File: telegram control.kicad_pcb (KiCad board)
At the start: 2 copper layers, 85.5 x 56 mm, 15 parts, among them J1 Screw_Terminal_01x03, J2 Screw_Terminal_01x02, K1 SANYOU_SRD_Form_C, Q1 MMBT3904, U1 ESP32-C3_SUPERMINI_TH, U3 L7805

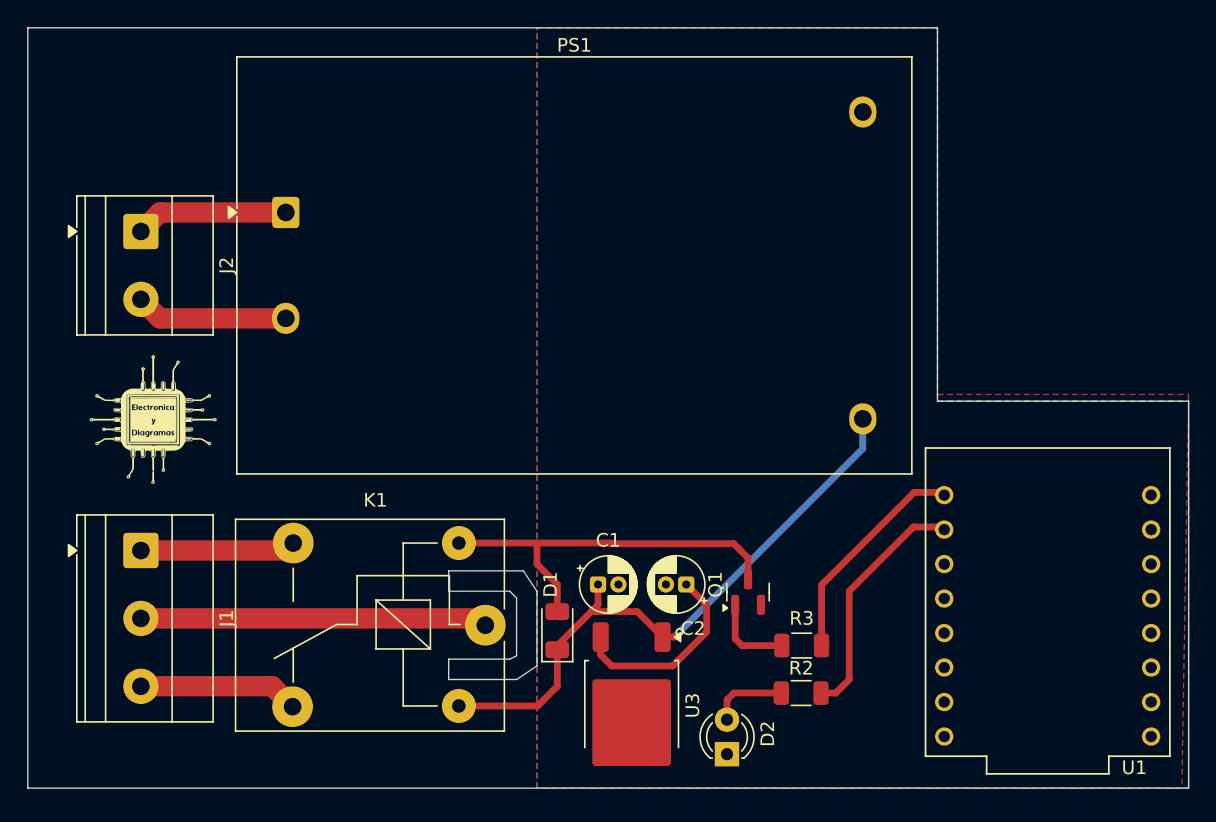
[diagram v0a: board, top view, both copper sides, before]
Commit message: telegram_control
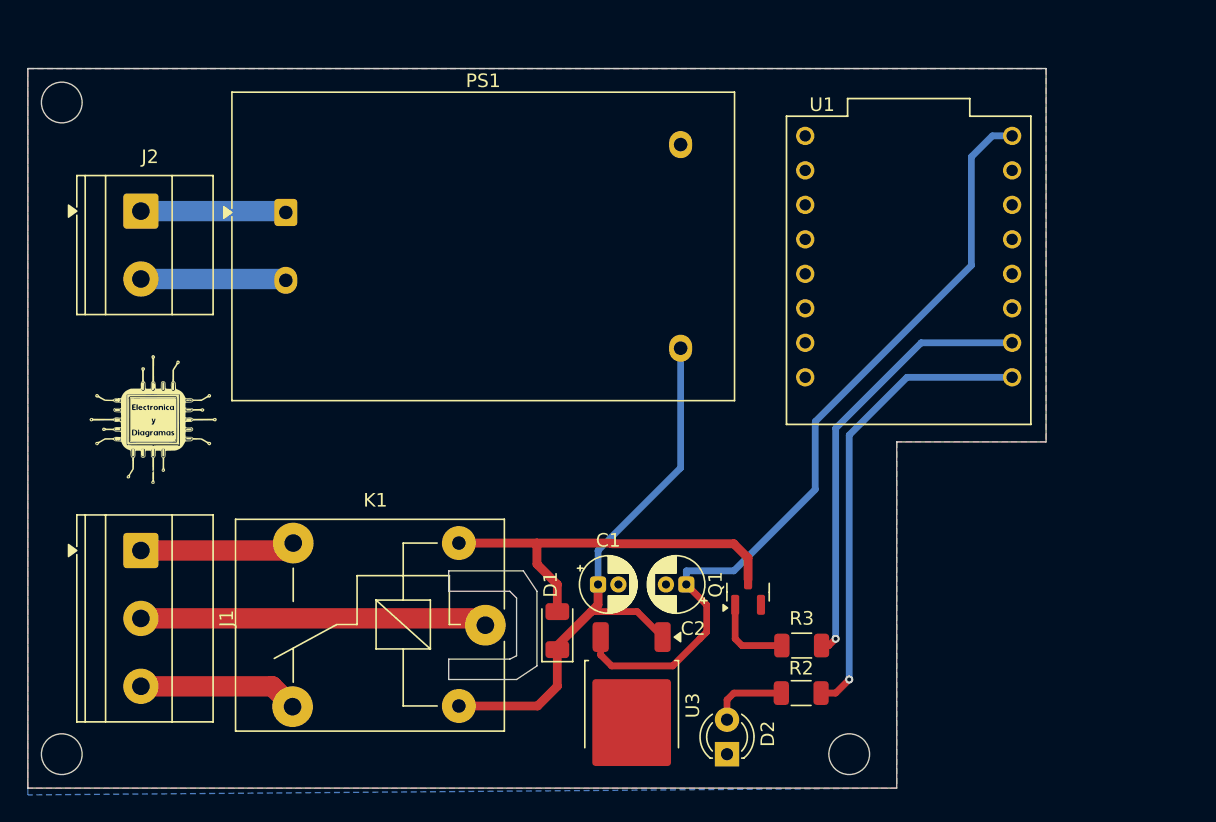
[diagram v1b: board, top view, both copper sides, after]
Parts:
- removed the G*** at (198.0, 89.0)
- added G***: LOGO, logo:logo_2, B.Cu at (188.0, 84.5)
- PS1: footprint Converter_ACDC:Converter_ACDC_Hi-Link_HLK-10Mxx -> Converter_ACDC:Converter_ACDC_Hi-Link_HLK-PMxx
- moved U1 26.5 mm to (219.9, 86.9), turned to 0 degrees
- moved J2 1.50 mm to (163.3, 82.5)
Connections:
- C2 pad 1: Net-(U3-OUT) -> +5V
- R2 pad 2: Net-(U1-GPIO1) -> Net-(U1-GPIO0)
- R3 pad 1: gpio0 -> gpio1
- U1 pad 0: gpio0 -> Net-(U1-GPIO0)
- U1 pad 1: Net-(U1-GPIO1) -> gpio1
- U3 pad 3: Net-(U3-OUT) -> +5V
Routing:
- net +5V: track 0.00 -> 60.5 mm
- net Net-(U1-GPIO0): track 0.00 -> 34.3 mm, vias 0 -> 1
- net gpio1: track 0.00 -> 32.4 mm, vias 0 -> 1
- net Net-(U1-GPIO1): track 18.2 -> 0.00 mm
- net gpio0: track 16.6 -> 0.00 mm
- net Net-(U3-OUT): track 14.6 -> 0.00 mm
- net +12V: track 45.3 -> 42.6 mm, vias 1 -> 0
- net Net-(J2-Pin_2): track 11.3 -> 10.7 mm
- net Net-(J2-Pin_1): track 11.3 -> 10.7 mm
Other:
- board size 85.5 x 56 mm -> 75 x 53 mm
